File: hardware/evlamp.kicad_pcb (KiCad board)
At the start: 2 copper layers, 56 x 63 mm, 25 parts, among them X1 LED 0, X10 DOWN, X11 MAIN, X2 LED 1, X3 LED 2, X4 LED 3, X5 LED 4, X6 LED 5, X7 LED 6, X8 LED 7, X9 UP

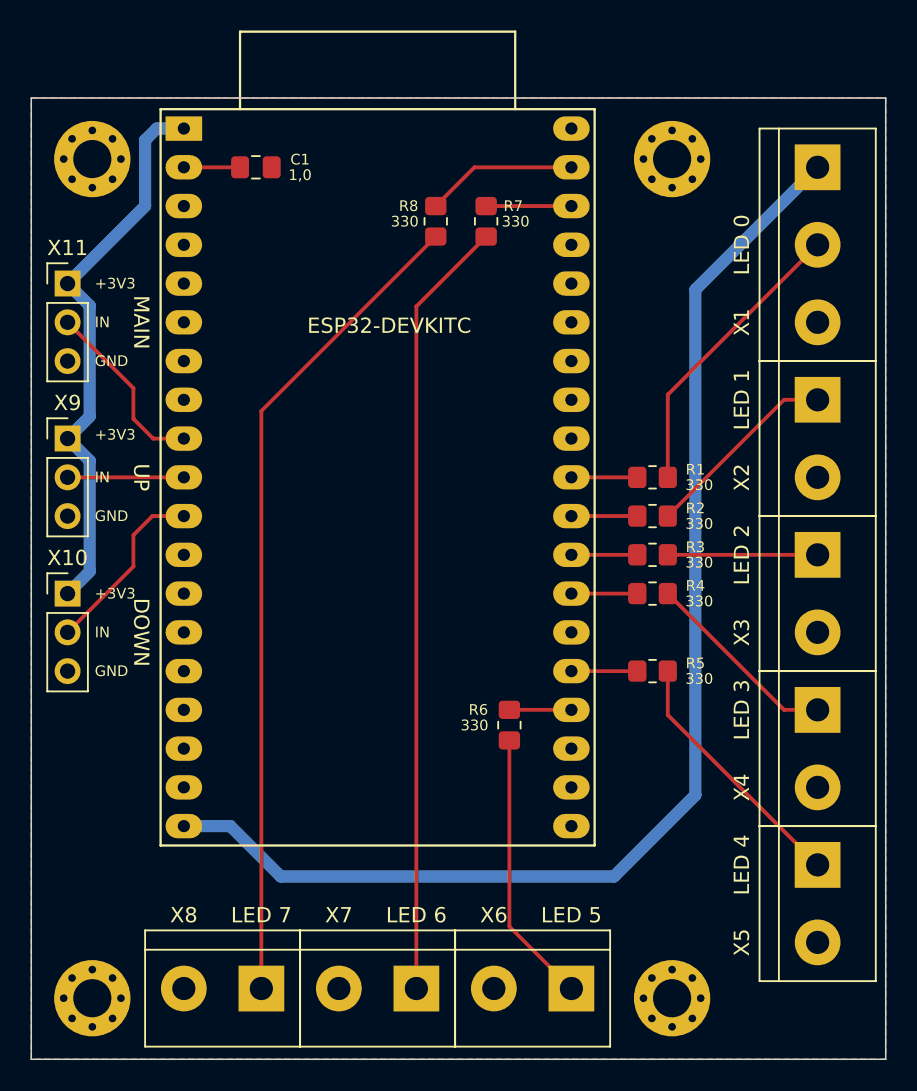
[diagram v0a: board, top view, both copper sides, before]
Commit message: update KiCad project
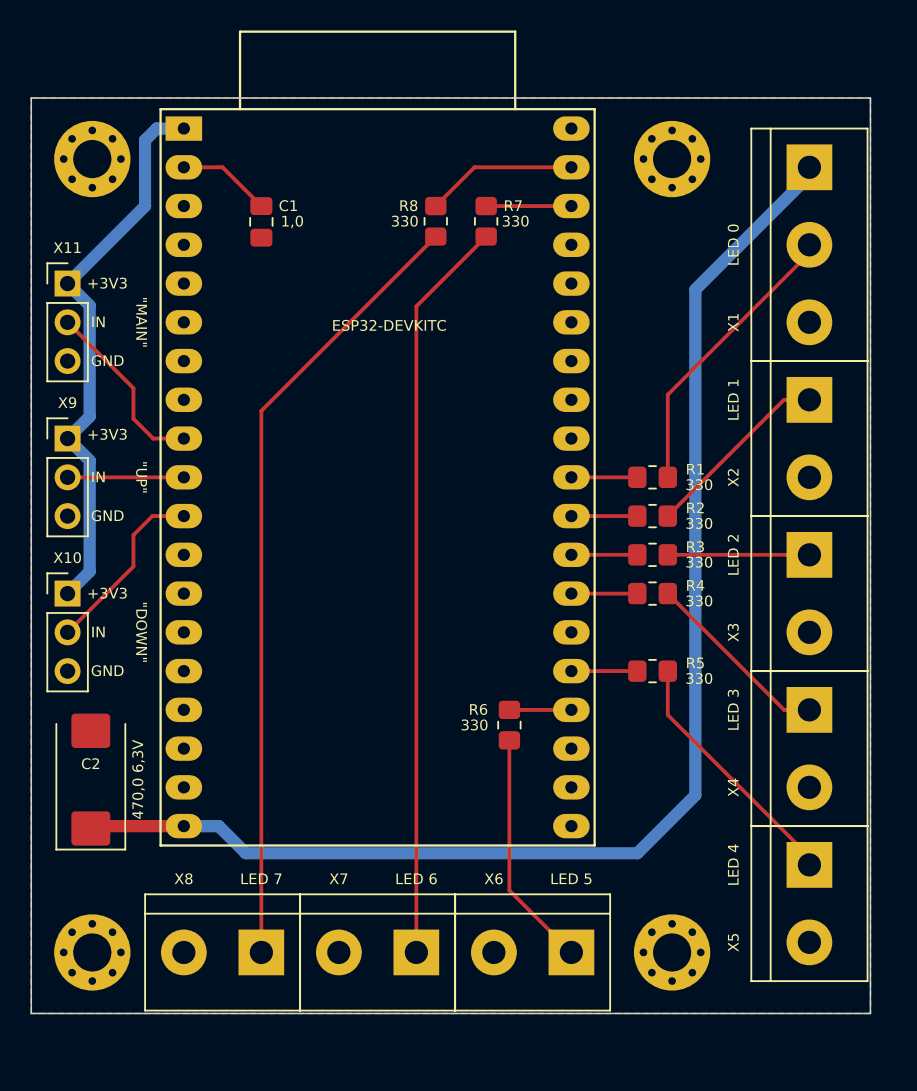
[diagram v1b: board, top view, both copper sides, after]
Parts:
- added C2: 470,0 6,3V, Capacitor_Tantalum_SMD:CP_EIA-7343-31_Kemet-D_Pad2.25x2.55mm_HandSolder, F.Cu at (76.5, 114.8)
- X10: value DOWN -> "DOWN"
- X11: value MAIN -> "MAIN"
- X9: value UP -> "UP"
- moved C1 3.60 mm to (87.6, 78.3), turned to 90 degrees
- moved REF** 3.00 mm to (76.5, 126.2)
- moved REF** 3.00 mm to (114.5, 126.2)
- moved X6 2.36 mm to (108.0, 126.2)
- moved X7 2.36 mm to (97.8, 126.2)
- moved X8 2.36 mm to (87.6, 126.2)
- moved X1 0.54 mm to (123.5, 74.7)
- moved X2 0.54 mm to (123.5, 89.9)
- moved X3 0.54 mm to (123.5, 100.1)
- moved X4 0.54 mm to (123.5, 110.3)
- moved X5 0.54 mm to (123.5, 120.4)
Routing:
- net +5V: track 81.6 -> 86.2 mm
- net Net-(C1-Pad2): track 3.68 -> 6.13 mm
- net Net-(R8-Pad2): track 54.0 -> 51.7 mm
- net Net-(R7-Pad2): track 51.2 -> 48.8 mm
- net Net-(R6-Pad2): track 17.9 -> 15.6 mm
- net Net-(R4-Pad2): track 13.0 -> 12.4 mm
- net Net-(R3-Pad2): track 9.82 -> 9.28 mm
- net Net-(R2-Pad2): track 13.0 -> 12.4 mm
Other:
- board size 56 x 63 mm -> 55 x 60 mm
